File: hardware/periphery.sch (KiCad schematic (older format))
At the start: 39 parts, among them J1 JAE_SIM_Card_SF72S006, J11 Micro_SD_Card_Ebay, J2 UART0, J3 Bus_PCI_Express_Mini, J8 HR911105_RJ45, U6 W25Q128JVS or W25N01GV, Y1 24MHz, Y2 32768

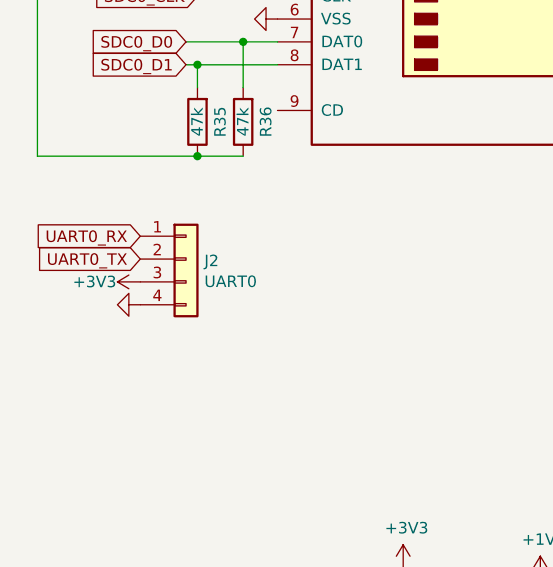
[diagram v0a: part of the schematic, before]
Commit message: Small touch-ups
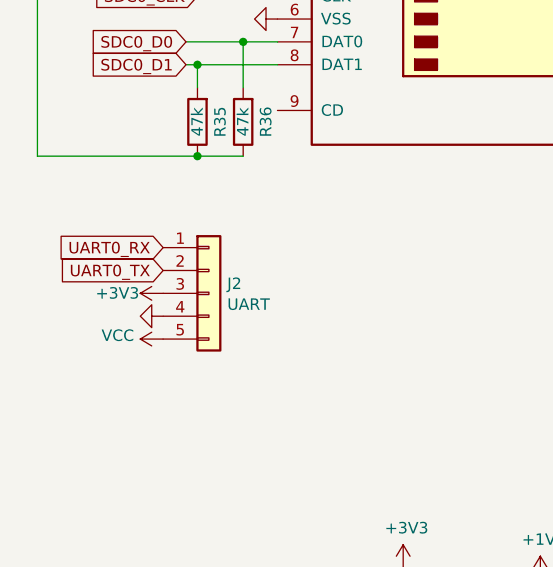
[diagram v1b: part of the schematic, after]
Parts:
- removed J2: UART0, Connector_PinSocket_1.27mm:PinSocket_1x04_P1.27mm_Vertical, symbol Connector_Generic:Conn_01x04
- added J2: UART, Connector_PinHeader_2.54mm:PinHeader_1x05_P2.54mm_Vertical, symbol Connector_Generic:Conn_01x05
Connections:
- net +3V3: now also J2.3 (Pin_3)
- net GND: now also J2.4 (Pin_4)
- net UART0_RX: now also J2.1 (Pin_1)
- net UART0_TX: now also J2.2 (Pin_2)
- new net VCC: J2.5 (Pin_5)
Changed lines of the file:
@@
-$EndComp
-$Comp
-L Connector_Generic:Conn_01x04 J2
-U 1 1 5F26BA8E
-P 1350 3200
-F 0 "J2" H 1430 3192 50  0000 L CNN
-F 1 "UART0" H 1430 3101 50  0000 L CNN
-F 2 "Connector_PinSocket_1.27mm:PinSocket_1x04_P1.27mm_Vertical" H 1350 3200 50  0001 C CNN
-F 3 "~" H 1350 3200 50  0001 C CNN
-	1    1350 3200
-	1    0    0    -1
 $EndComp
 $Comp
 L power:GND #PWR0182
 U 1 1 5F270335
-P 1150 3400
-F 0 "#PWR0182" H 1150 3150 50  0001 C CNN
-F 1 "GND" H 1155 3227 50  0001 C CNN
-F 2 "" H 1150 3400 50  0001 C CNN
-F 3 "" H 1150 3400 50  0001 C CNN
-	1    1150 3400
+P 1250 3450
+F 0 "#PWR0182" H 1250 3200 50  0001 C CNN
+F 1 "GND" H 1255 3277 50  0001 C CNN
+F 2 "" H 1250 3450 50  0001 C CNN
+F 3 "" H 1250 3450 50  0001 C CNN
+	1    1250 3450
 	0    1    1    0
 $EndComp
@@
 Text GLabel 1150 5300 0    50   Input ~ 0
 USB-D-
-Text GLabel 1150 3200 0    50   Input ~ 0
+Text GLabel 1250 3250 0    50   Input ~ 0
 UART0_TX
 $Comp
 L power:+3V3 #PWR0181
 U 1 1 5F27004D
-P 1150 3300
-F 0 "#PWR0181" H 1150 3150 50  0001 C CNN
-F 1 "+3V3" V 1150 3500 50  0000 C CNN
-F 2 "" H 1150 3300 50  0001 C CNN
-F 3 "" H 1150 3300 50  0001 C CNN
-	1    1150 3300
+P 1250 3350
+F 0 "#PWR0181" H 1250 3200 50  0001 C CNN
+F 1 "+3V3" V 1250 3550 50  0000 C CNN
+F 2 "" H 1250 3350 50  0001 C CNN
+F 3 "" H 1250 3350 50  0001 C CNN
+	1    1250 3350
 	0    -1   -1   0
 $EndComp
-Text GLabel 1150 3100 0    50   Input ~ 0
+Text GLabel 1250 3150 0    50   Input ~ 0
 UART0_RX
 $Comp
@@
 Text Label 1600 5300 0    50   ~ 0
 USB_H-D-
+$Comp
+L power:VCC #PWR0176
+U 1 1 62786CAF
+P 1250 3550
+F 0 "#PWR0176" H 1250 3400 50  0001 C CNN
+F 1 "VCC" V 1265 3677 50  0000 L CNN
+F 2 "" H 1250 3550 50  0001 C CNN
+F 3 "" H 1250 3550 50  0001 C CNN
+	1    1250 3550
+	0    -1   -1   0
+$EndComp
+$Comp
+L Connector_Generic:Conn_01x05 J2
+U 1 1 6279ABFA
+P 1450 3350
+F 0 "J2" H 1530 3392 50  0000 L CNN
+F 1 "UART" H 1530 3301 50  0000 L CNN
+F 2 "Connector_PinHeader_2.54mm:PinHeader_1x05_P2.54mm_Vertical" H 1450 3350 50  0001 C CNN
+F 3 "~" H 1450 3350 50  0001 C CNN
+	1    1450 3350
+	1    0    0    -1
+$EndComp
 $EndSCHEMATC
